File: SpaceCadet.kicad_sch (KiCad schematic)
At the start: 35 parts, among them J0 Conn_02x17_Odd_Even, J3_1 Conn_01x04, J3_2 Conn_01x04, U1 74LS154, U2 8048, Y3 Crystal 3.58MHz

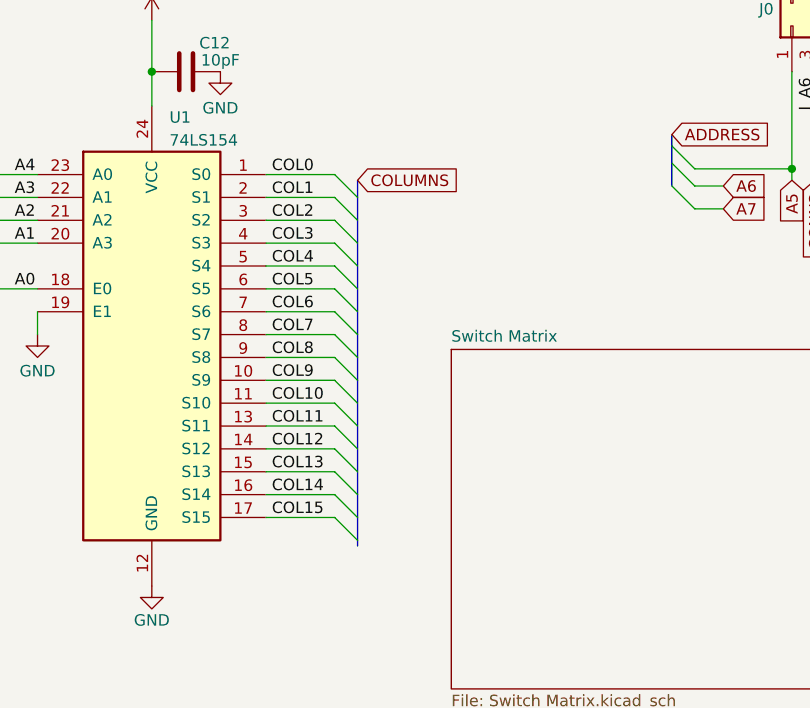
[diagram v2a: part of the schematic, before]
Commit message: wip: columns preparing
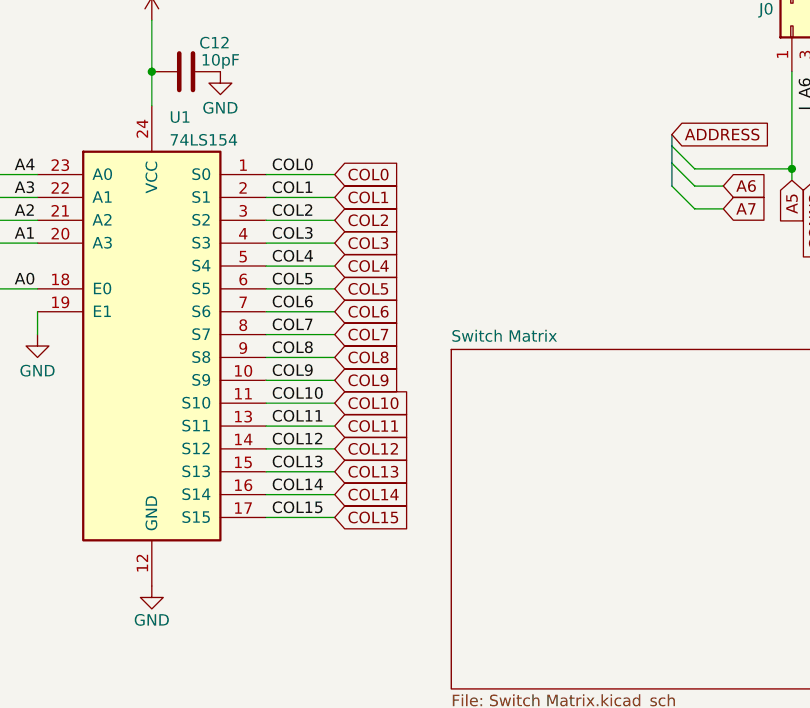
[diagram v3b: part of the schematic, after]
